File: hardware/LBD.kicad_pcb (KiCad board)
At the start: 2 copper layers, 13.4 x 46.9 mm, 10 parts, among them J2 USB4155-03-C_REVA, U1 RP2040, U4 TPSM828214SILR

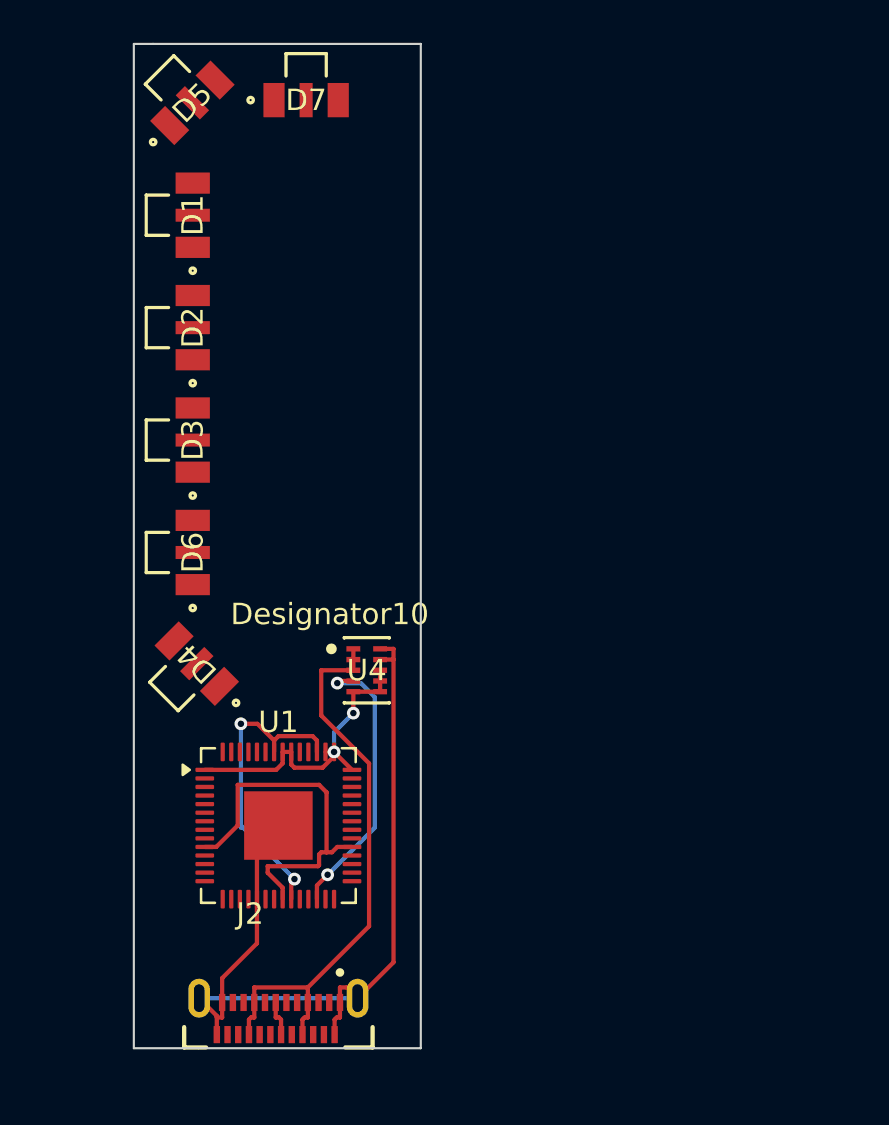
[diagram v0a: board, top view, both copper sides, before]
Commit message: feat: place components
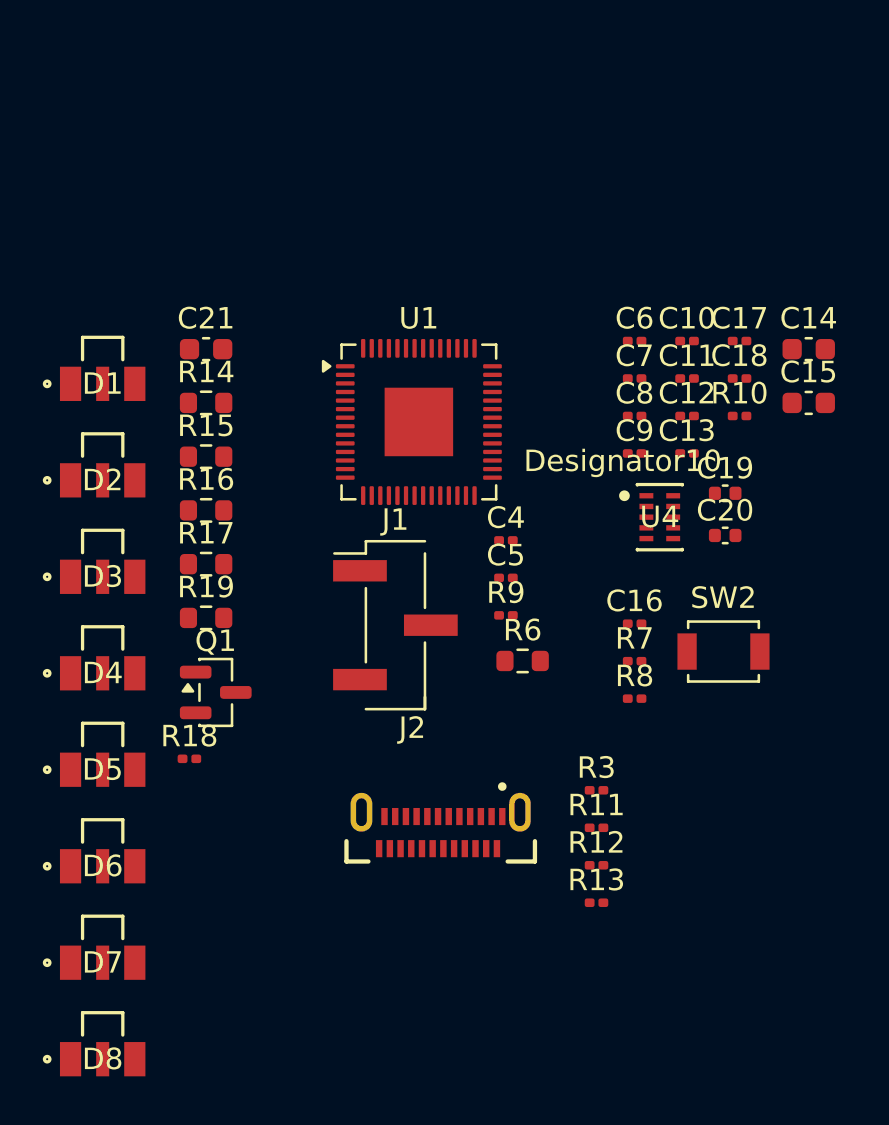
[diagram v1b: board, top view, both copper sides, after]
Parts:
- added C10: 100n, Capacitor_SMD:C_0201_0603Metric, F.Cu at (166.1, 92.4)
- added C11: 100n, Capacitor_SMD:C_0201_0603Metric, F.Cu at (166.1, 94.1)
- added C12: 100n, Capacitor_SMD:C_0201_0603Metric, F.Cu at (166.1, 95.9)
- added C13: 100n, Capacitor_SMD:C_0201_0603Metric, F.Cu at (166.1, 97.6)
- added C14: 4.7u, Capacitor_SMD:C_0603_1608Metric, F.Cu at (171.8, 92.8)
- added C15: 22u, Capacitor_SMD:C_0603_1608Metric, F.Cu at (171.8, 95.3)
- added C16: 100n, Capacitor_SMD:C_0201_0603Metric, F.Cu at (163.6, 105.6)
- added C17: 100n, Capacitor_SMD:C_0201_0603Metric, F.Cu at (168.5, 92.4)
- added C18: 100n, Capacitor_SMD:C_0201_0603Metric, F.Cu at (168.5, 94.1)
- added C19: 1u, Capacitor_SMD:C_0402_1005Metric, F.Cu at (167.9, 99.5)
- added C20: 1u, Capacitor_SMD:C_0402_1005Metric, F.Cu at (167.9, 101.5)
- added C21: 10u, Capacitor_SMD:C_0603_1608Metric, F.Cu at (143.6, 92.8)
- added C4: 15p, Capacitor_SMD:C_0201_0603Metric, F.Cu at (157.6, 101.7)
- added C5: 15p, Capacitor_SMD:C_0201_0603Metric, F.Cu at (157.6, 103.4)
- added C6: 100n, Capacitor_SMD:C_0201_0603Metric, F.Cu at (163.6, 92.4)
- added C7: 100n, Capacitor_SMD:C_0201_0603Metric, F.Cu at (163.6, 94.1)
- added C8: 100n, Capacitor_SMD:C_0201_0603Metric, F.Cu at (163.6, 95.9)
- added C9: 100n, Capacitor_SMD:C_0201_0603Metric, F.Cu at (163.6, 97.6)
- added D8: IN-S126ESGHIR, LBD_Footprints:LED_IN-S12_INL, F.Cu at (138.8, 125.9)
- added J1: Conn_01x03_Pin, Connector_PinHeader_2.54mm:PinHeader_1x03_P2.54mm_Vertical_SMD_Pin1Left, F.Cu at (152.5, 105.6)
- added Q1: AO3400A, Package_TO_SOT_SMD:SOT-23, F.Cu at (144.1, 108.8)
- added R10: 100k, Resistor_SMD:R_0201_0603Metric, F.Cu at (168.5, 95.9)
- added R11: 22, Resistor_SMD:R_0201_0603Metric, F.Cu at (161.9, 115.1)
- added R12: 22, Resistor_SMD:R_0201_0603Metric, F.Cu at (161.9, 116.9)
- added R13: 5.1k, Resistor_SMD:R_0201_0603Metric, F.Cu at (161.9, 118.6)
- added R14: 22, Resistor_SMD:R_0603_1608Metric, F.Cu at (143.6, 95.3)
- added R15: 22, Resistor_SMD:R_0603_1608Metric, F.Cu at (143.6, 97.8)
- added R16: 22, Resistor_SMD:R_0603_1608Metric, F.Cu at (143.6, 100.3)
- added R17: 22, Resistor_SMD:R_0603_1608Metric, F.Cu at (143.6, 102.8)
- added R18: 10k, Resistor_SMD:R_0201_0603Metric, F.Cu at (142.8, 111.9)
- added R19: 33, Resistor_SMD:R_0603_1608Metric, F.Cu at (143.6, 105.3)
- added R3: 5.1k, Resistor_SMD:R_0201_0603Metric, F.Cu at (161.9, 113.4)
- added R6: 1k (0603), Resistor_SMD:R_0603_1608Metric, F.Cu at (158.4, 107.3)
- added R7: 1k, Resistor_SMD:R_0201_0603Metric, F.Cu at (163.6, 107.3)
- added R8: 10k, Resistor_SMD:R_0201_0603Metric, F.Cu at (163.6, 109.1)
- added R9: 10k, Resistor_SMD:R_0201_0603Metric, F.Cu at (157.6, 105.2)
- added SW2: BOOTSEL, Button_Switch_SMD:SW_SPST_B3U-1000P, F.Cu at (167.8, 106.9)
- D1, D2, D3, D4, D5, D6, D7: value LED -> IN-S126ESGHIR
- J2: value USB4155-03-C_REVA -> USB4155-03-C
- moved D7 41.4 mm to (138.8, 121.4)
- moved D5 31.4 mm to (138.8, 112.4), turned to 0 degrees
- moved U1 20.0 mm to (153.6, 96.2)
- moved U4 15.4 mm to (164.8, 100.6)
- moved D6 15.2 mm to (138.8, 116.9), turned to 0 degrees
- moved J2 11.5 mm to (154.6, 115.3)
- moved D1 8.93 mm to (138.8, 94.4), turned to 0 degrees
- moved D2 8.28 mm to (138.8, 98.9), turned to 0 degrees
- moved D3 7.65 mm to (138.8, 103.4), turned to 0 degrees
- moved D4 4.42 mm to (138.8, 107.9), turned to 0 degrees
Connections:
- D1 pad 1: unconnected-(D1-K-Pad1) -> Net-(D1-K)
- D1 pad 2: unconnected-(D1-A-Pad2) -> Net-(D1-A)
- D2 pad 1: unconnected-(D2-K-Pad1) -> Net-(D2-K)
- D2 pad 2: unconnected-(D2-A-Pad2) -> Net-(D2-A)
- D3 pad 1: unconnected-(D3-K-Pad1) -> Net-(D3-K)
- D3 pad 2: unconnected-(D3-A-Pad2) -> Net-(D3-A)
- D4 pad 1: unconnected-(D4-K-Pad1) -> Net-(D4-K)
- D4 pad 2: unconnected-(D4-A-Pad2) -> Net-(D4-A)
- D5 pad 1: unconnected-(D5-K-Pad1) -> Net-(D5-K)
- D5 pad 2: unconnected-(D5-A-Pad2) -> Net-(D1-K)
- D6 pad 1: unconnected-(D6-K-Pad1) -> Net-(D5-K)
- D6 pad 2: unconnected-(D6-A-Pad2) -> Net-(D2-K)
- D7 pad 1: unconnected-(D7-K-Pad1) -> Net-(D5-K)
- D7 pad 2: unconnected-(D7-A-Pad2) -> Net-(D3-K)
- U1 pad 4: unconnected-(U1-GPIO2-Pad4) -> /Infared/IR_GATE
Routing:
- net GND: track 41.4 -> 0.00 mm
- net +3.3V: track 32.2 -> 0.00 mm, vias 2 -> 0
- net VBUS: track 26.7 -> 0.00 mm
- net +1V1: track 14.5 -> 0.00 mm, vias 2 -> 0
- net /Power/PG: track 13.4 -> 0.00 mm, vias 2 -> 0
- net /USB/DN: track 1.69 -> 0.00 mm
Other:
- board outline removed
